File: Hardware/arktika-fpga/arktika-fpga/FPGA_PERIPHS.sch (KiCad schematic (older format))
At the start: 22 parts

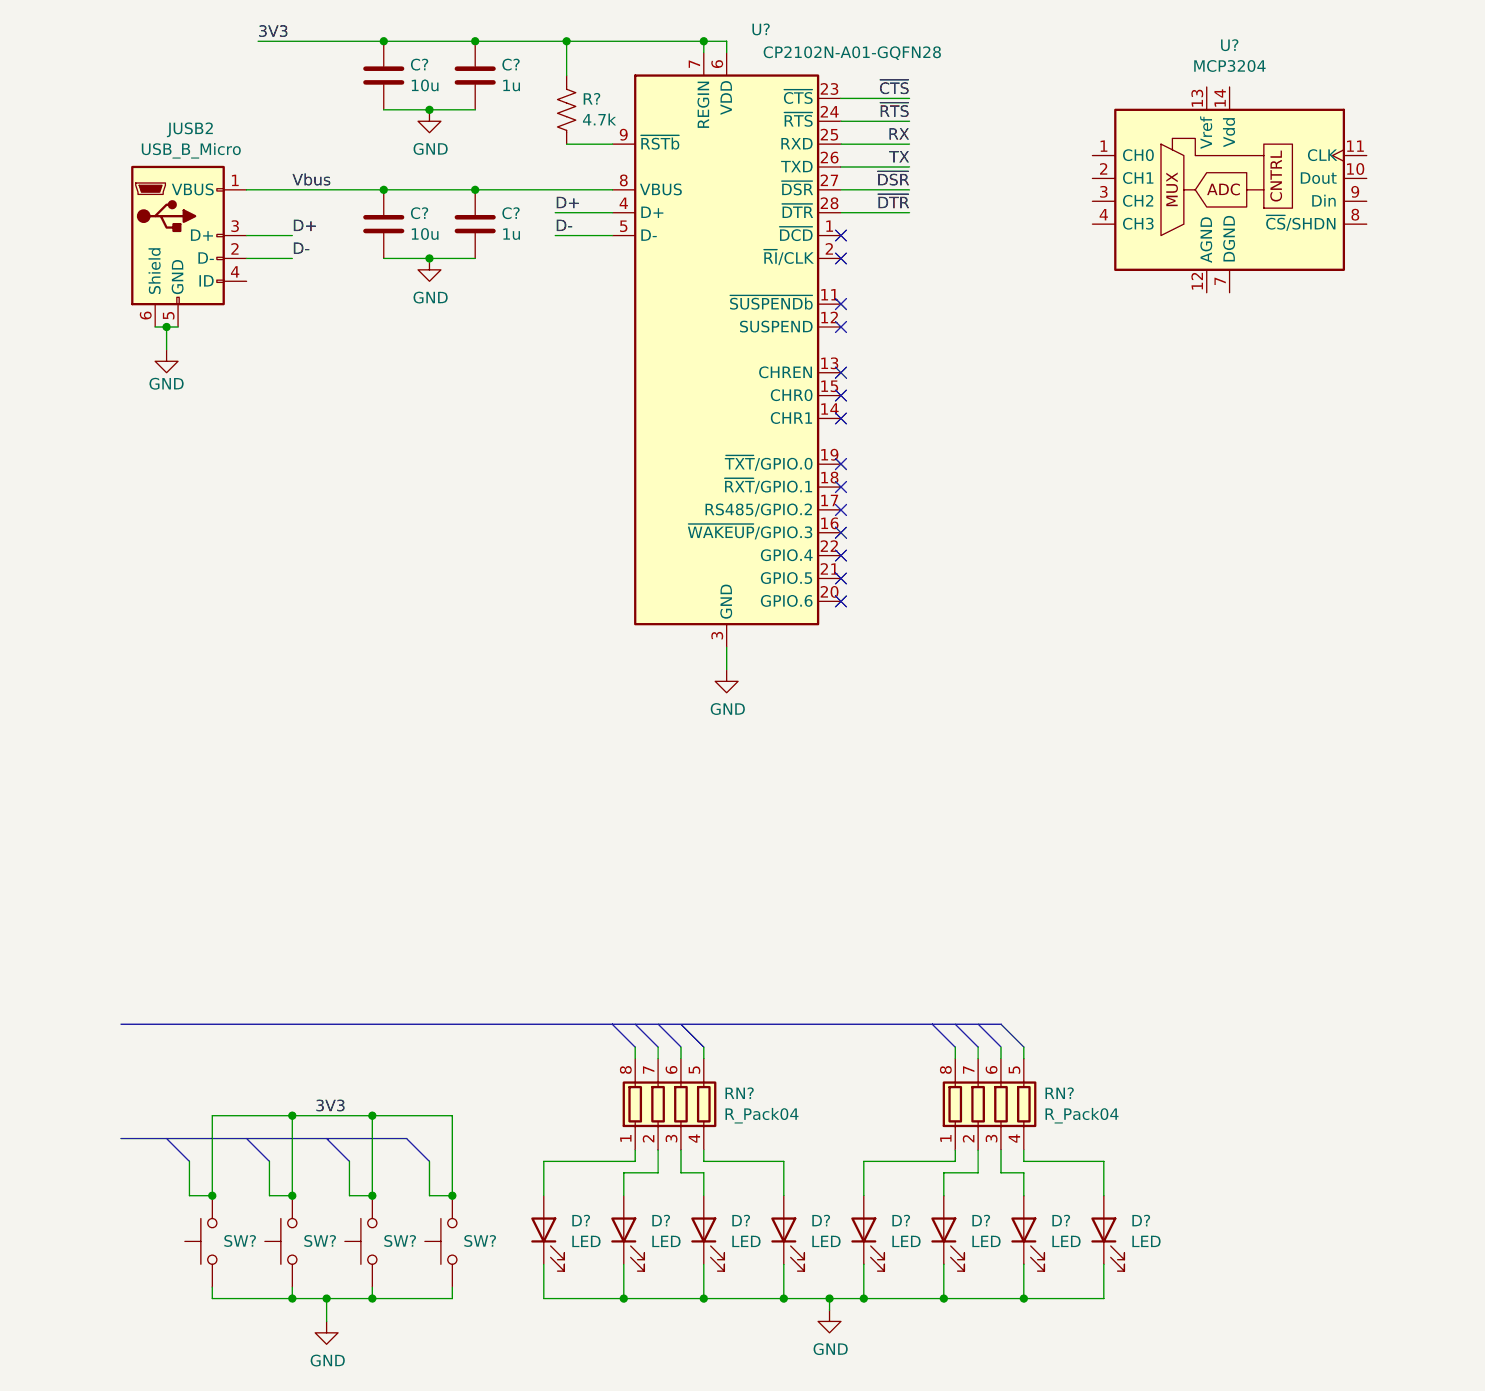
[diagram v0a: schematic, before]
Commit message: Minor fixes
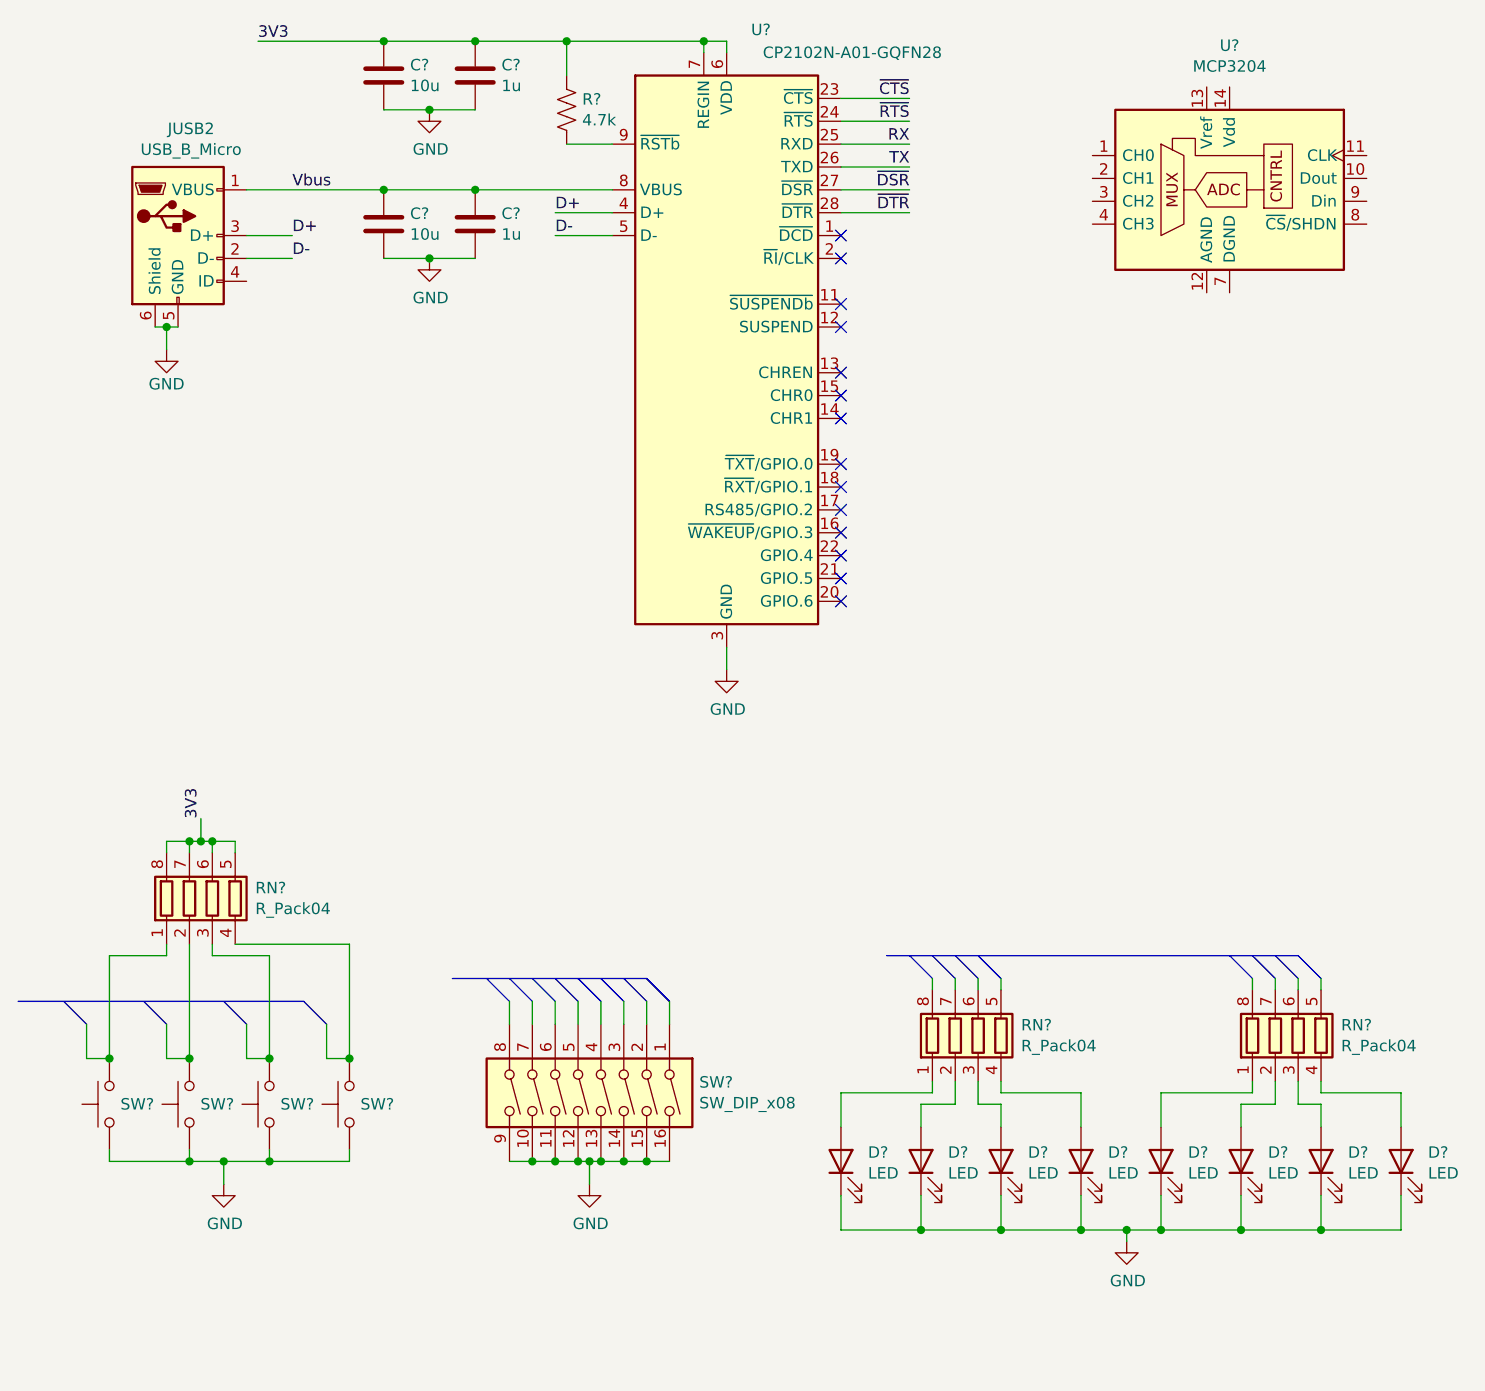
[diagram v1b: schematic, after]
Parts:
- added RN?: R_Pack04, symbol Device:R_Pack04
- added SW?: SW_DIP_x08, symbol Switch:SW_DIP_x08
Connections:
- wire segments 103 -> 131
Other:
- moved on the sheet: D?, RN?, SW?
